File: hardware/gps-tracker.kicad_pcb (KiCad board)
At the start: 4 copper layers, 87.6 x 80.9 mm, 95 parts, among them J1 USB_B_Micro, J2 Conn_01x07, J3 Conn_01x08, J4 Conn_01x03, J5 Conn_01x04, SW1 SW_Push, SW2 SW_Push, SW3 SW_Push, SW4 SW_Push, SW5 SW_Push, SW6 SW_SPDT, U1 STM32G070KBTx, U2 CH340C, U3 LTR-303ALS-01, U4 MIC5365-3.3YD5, U5 LIS2MDLTR, U6 LC86LICMD, U7 E22-900M22S, U8 TP4056, U9 MIC5365-3.3YD5

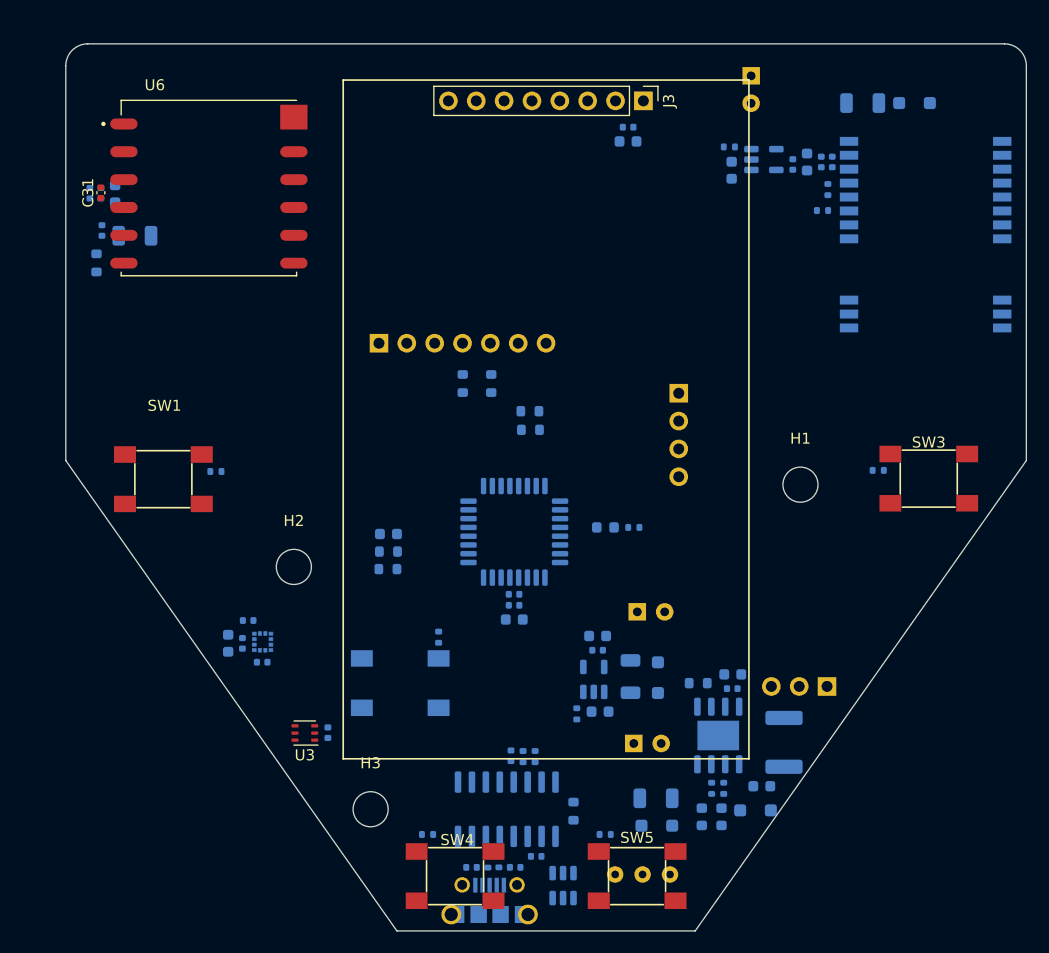
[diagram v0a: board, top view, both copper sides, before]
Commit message: Hardware v1.0
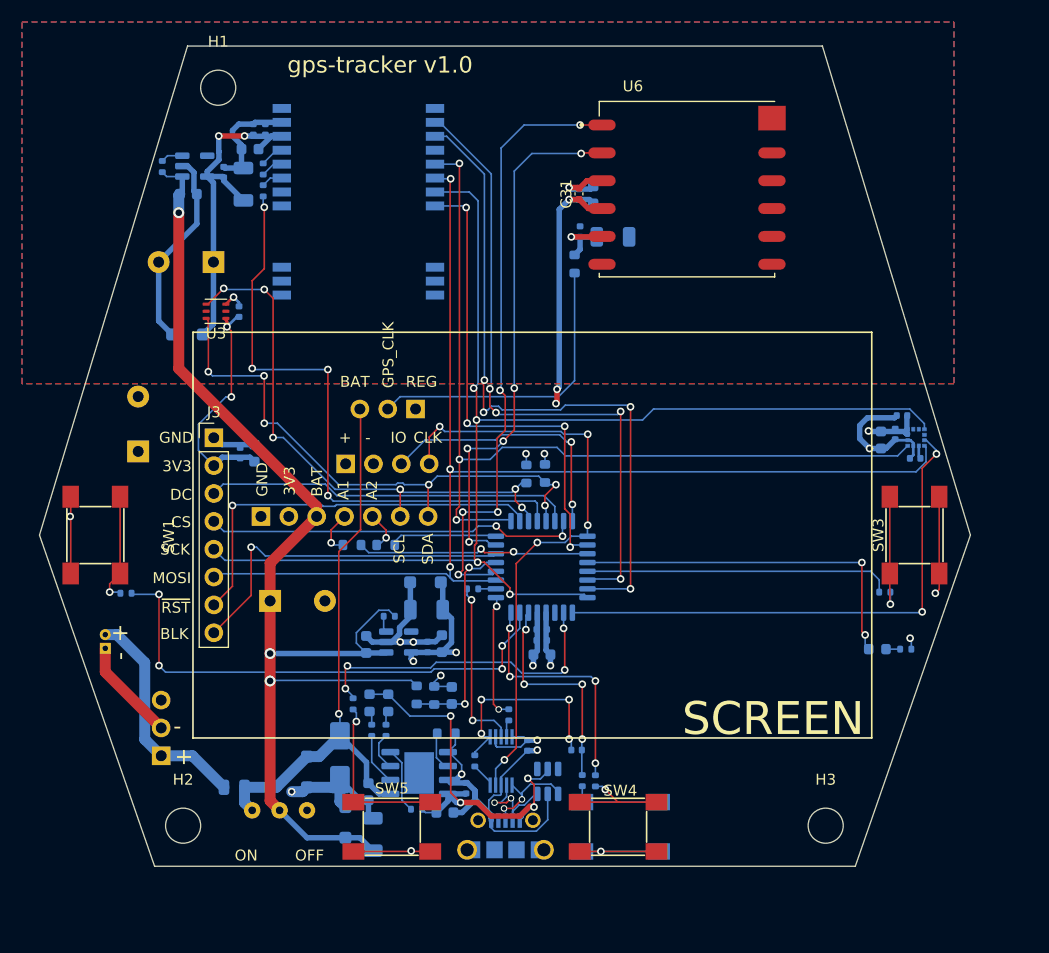
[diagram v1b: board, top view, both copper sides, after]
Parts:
- removed C13: 10uF, Capacitor_SMD:C_0603_1608Metric
- removed C38: 470uF, Homebrew:CP_Radial_D6.3mm_P2.50mm_470uF
- removed R9: 22, Resistor_SMD:R_0402_1005Metric
- added D9: D, Diode_SMD:D_SMA, B.Cu at (96.0, 117.1)
- added J6: Conn_01x03, Connector_PinHeader_2.54mm:PinHeader_1x03_P2.54mm_Vertical, B.Cu at (102.9, 85.3)
- added J7: Conn_01x02, Homebrew:JST_Micro_1x02_P1.25mm_Horizontal, B.Cu at (74.6, 106.5)
- C16, C19: value 470uF -> 220uF; footprint Homebrew:CP_Radial_D6.3mm_P2.50mm_470uF -> Capacitor_THT:CP_Radial_D10.0mm_P5.00mm
- C2: value 47pF -> 10uF; footprint Capacitor_SMD:C_0402_1005Metric -> Capacitor_SMD:C_0603_1608Metric
- C3: value 47pF -> 220uF; footprint Capacitor_SMD:C_0402_1005Metric -> Capacitor_THT:CP_Radial_D10.0mm_P5.00mm
- R2: value 3k3 -> 220; footprint Resistor_SMD:R_0603_1608Metric -> Resistor_SMD:R_0402_1005Metric
- R4: value 22 -> 4k7
- R6: value 22 -> 1k
- R8: value 22 -> 220
- TH1: footprint Fuse:Fuse_1812_4532Metric_Pad1.30x3.40mm_HandSolder -> Fuse:Fuse_0805_2012Metric
- U2: value CH340C -> CH340X; footprint Package_SO:SOIC-16_3.9x9.9mm_P1.27mm -> Package_SO:MSOP-10_3x3mm_P0.5mm
- moved D8 69.6 mm to (82.1, 78.5), turned to 180 degrees
- moved H1 64.3 mm to (84.9, 56.0)
- moved C17 62.5 mm to (146.6, 87.6)
- moved C20 62.5 mm to (147.3, 85.9)
- moved U5 62.4 mm to (148.5, 87.9)
- moved C18 62.4 mm to (148.5, 89.8)
- moved C35 62.4 mm to (145.3, 88.1)
- moved C3 61.7 mm to (84.5, 71.9), turned to 180 degrees
- moved J4 61.1 mm to (79.7, 116.9), turned to 0 degrees
- moved C37 57.0 mm to (87.2, 64.8), turned to -90 degrees
- moved C19 52.5 mm to (77.6, 89.2), turned to 90 degrees
- moved C36 51.9 mm to (85.4, 63.7)
- moved U9 51.9 mm to (82.8, 63.1)
- moved C25 51.9 mm to (88.1, 59.8)
- moved U7 51.8 mm to (90.7, 74.9)
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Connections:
- net /GPS_RXD renamed /GPS_TX
- net /GPS_TXD renamed /GPS_RX
- net /USART_TXD renamed /USART_RX
- C16 pad 1: VCC -> +BATT
- C19 pad 1: +BATT -> VCC
- C2 pad 1: /USB+ -> GND
- C2 pad 2: GND -> /BATT_DIRECT
- C3 pad 1: /USB- -> /RADIO_PWR
- D7 pad 2: Net-(D7-A) -> VBUS
- R2 pad 1: /BOOT0 -> Net-(U2-RXD)
- R2 pad 2: VBUS -> /USART_TX
- R21 pad 2: VCC -> Net-(J6-Pin_2)
- R4 pad 1: /USB+ -> Net-(U2-~{CTS})
- R4 pad 2: Net-(U2-UD+) -> /~{DTR}
- R6 pad 1: /USB- -> VBUS
- R6 pad 2: Net-(U2-UD-) -> Net-(U8-CE)
- SW6 pad 1: /BATT_DIRECT -> unconnected-(SW6-A-Pad1)
- SW6 pad 3: unconnected-(SW6-C-Pad3) -> /BATT_DIRECT
- U1 pad 2: /RADIO_RXEN -> /SW4
- U1 pad 20: /SW4 -> /RADIO_RXEN
- U1 pad 26: unconnected-(U1-PA15-Pad26) -> /RADIO_CS
- U1 pad 29: /SW1 -> /SW2
- U1 pad 3: /RADIO_CS -> unconnected-(U1-PC15-Pad3)
- U1 pad 7: /SW2 -> /SW1
- U1 pad 9: /USART_RXD -> /USART_TX
- U2 pad 1: GND -> /USB+
- U2 pad 10: unconnected-(U2-~{DSR}-Pad10) -> VCC
- U2 pad 2: Net-(U2-TXD) -> /USB-
- U2 pad 3: Net-(U2-RXD) -> GND
- U2 pad 4: VCC -> /BOOT0
- U2 pad 5: Net-(U2-UD+) -> Net-(U2-~{CTS})
- U2 pad 6: Net-(U2-UD-) -> /~{DTR}
- U2 pad 7: unconnected-(U2-NC-Pad7) -> VCC
- U2 pad 8: unconnected-(U2-NC-Pad8) -> Net-(U2-TXD)
- U2 pad 9: unconnected-(U2-~{CTS}-Pad9) -> Net-(U2-RXD)
- U8 pad 8: Net-(D7-A) -> Net-(U8-CE)
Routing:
- net GND: track 0.00 -> 166.7 mm, vias 0 -> 15
- net /SCK: track 0.00 -> 116.3 mm, vias 0 -> 4
- net /MOSI: track 0.00 -> 109.1 mm, vias 0 -> 3
- net +BATT: track 0.00 -> 108.2 mm, vias 0 -> 3
- net /MISO: track 0.00 -> 81.8 mm, vias 0 -> 3
- net VCC: track 0.00 -> 76.5 mm, vias 0 -> 12
- net /RADIO_BUSY: track 0.00 -> 62.2 mm, vias 0 -> 4
- net /RADIO_DIO1: track 0.00 -> 58.2 mm, vias 0 -> 4
- net /GPS_TX: track 0.00 -> 56.5 mm, vias 0 -> 5
- net /RADIO_RXEN: track 0.00 -> 55.6 mm, vias 0 -> 4
- net /BOOT0: track 0.00 -> 55.4 mm, vias 0 -> 5
- net /BATT_DIRECT: track 0.00 -> 51.3 mm, vias 0 -> 1
- net /SDA: track 0.00 -> 50.6 mm, vias 0 -> 6
- net /SCL: track 0.00 -> 50.4 mm, vias 0 -> 6
- net /COMPASS_CS: track 0.00 -> 48.7 mm, vias 0 -> 2
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- added copper zone on B.Cu, net GND
- added copper zone on F.Cu, net GND
- added copper zone on In1.Cu, net GND
- added copper zone on In2.Cu, net GND
- added copper zone on In1.Cu, net VCC
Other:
- board size 87.6 x 80.9 mm -> 84.9 x 74.8 mm
- board text added: "+"
- board text added: "-"
- board text added: "2Ah BATTERY"
- board text added: "3V3"
- board text added: "A1"
- board text added: "A2"
- board text added: "BAT"
- board text added: "BLK"
- board text added: "CHARGE"
- board text added: "CLK"
- board text added: "CS"
- board text added: "DC"
- board text added: "GND"
- board text added: "GPS_CLK"
- board text added: "IO"
- board text added: "MOSI"
- board text added: "OFF"
- board text added: "ON"
- board text added: "REG"
- board text added: "RESET"
- board text added: "SCK"
- board text added: "SCL"
- board text added: "SCREEN"
- board text added: "SDA"
- board text added: "gps-tracker v1.0"
- board text added: "~{RST}"
